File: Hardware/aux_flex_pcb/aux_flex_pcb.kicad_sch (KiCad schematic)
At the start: 17 parts, among them U1 STM32L432KCUx

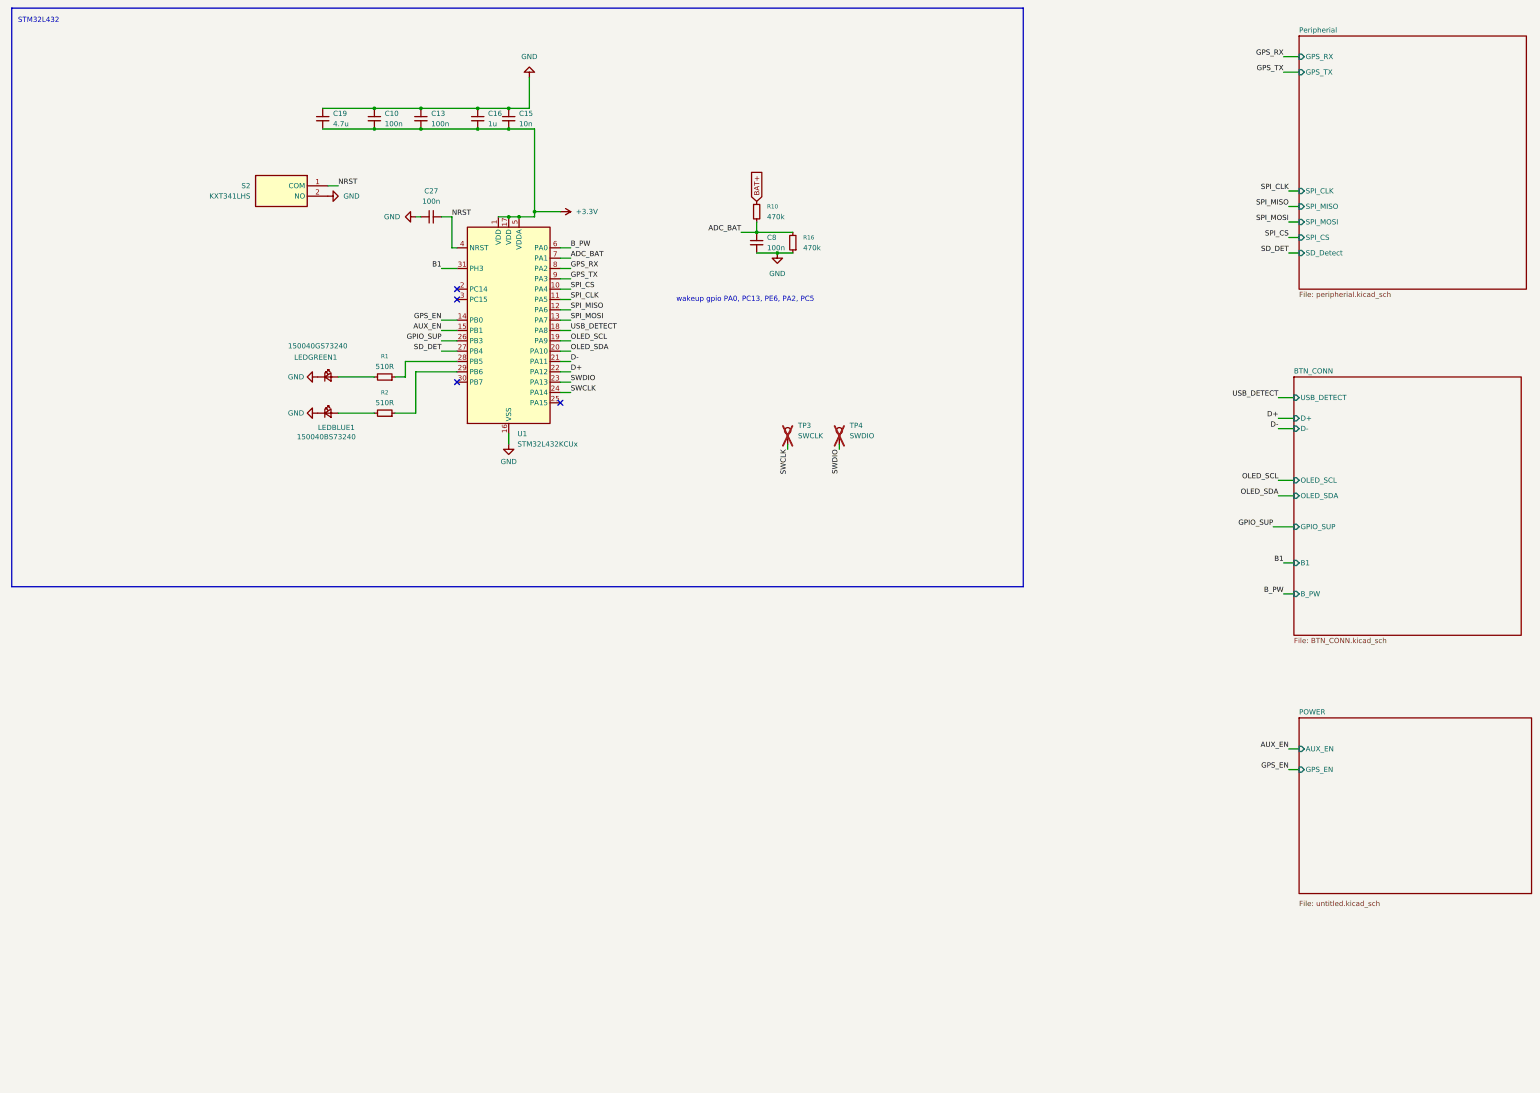
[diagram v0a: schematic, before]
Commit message: up
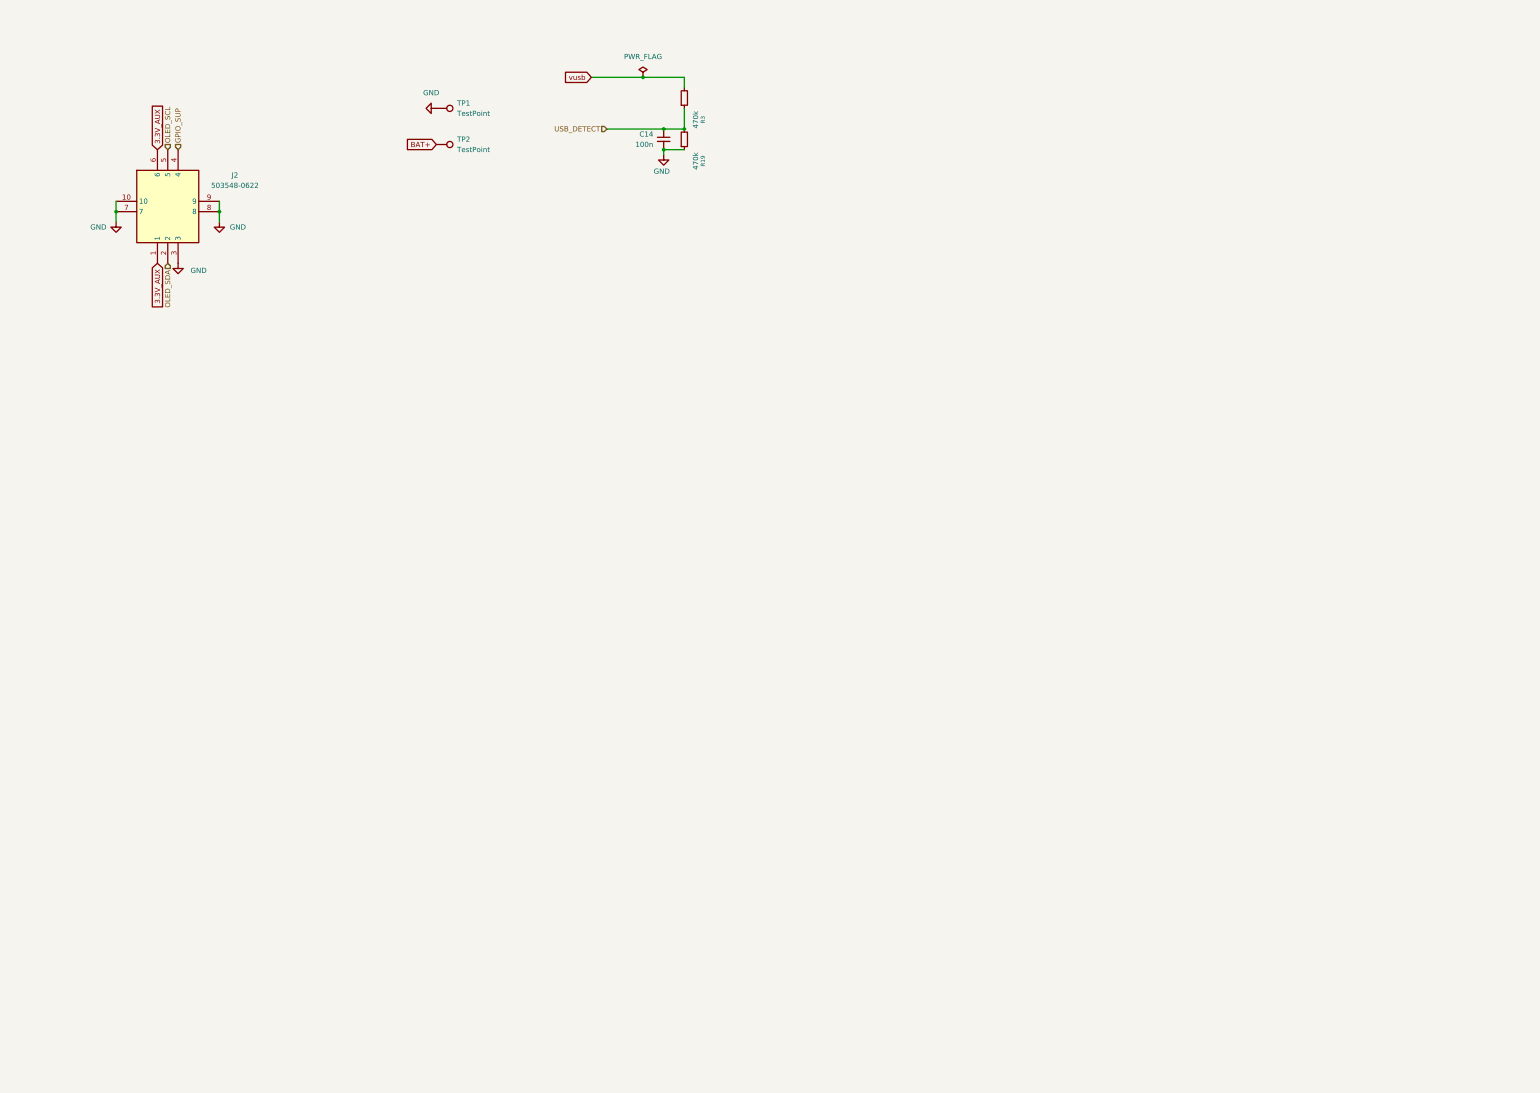
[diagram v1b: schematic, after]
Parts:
- removed C10, C13, C27, C8: 100n, v9footprint:C_0201_0603Metric_Pad0.64x0.40mm_HandSolder, symbol Device:C_Small
- removed C15: 10n, v9footprint:C_0201_0603Metric_Pad0.64x0.40mm_HandSolder, symbol Device:C_Small
- removed C16: 1u, v9footprint:C_0201_0603Metric_Pad0.64x0.40mm_HandSolder, symbol Device:C_Small
- removed C19: 4.7u, v9footprint:C_0402_1005Metric, symbol Device:C_Small
- removed LEDBLUE1: 150040BS73240, v9footprint:LED_0402_1005Metric, symbol Device:LED_Small
- removed LEDGREEN1: 150040GS73240, v9footprint:LED_0402_1005Metric, symbol Device:LED_Small
- removed R1, R2: 510R, v9footprint:R_0201_0603Metric_Pad0.64x0.40mm_HandSolder, symbol Device:R_Small
- removed R10, R16: 470k, v9footprint:R_0201_0603Metric_Pad0.64x0.40mm_HandSolder, symbol Device:R_Small
- removed S2: KXT341LHS, v9footprint:KXT341LHS, symbol samacsys:KXT341LHS
- removed TP3: SWCLK, v9footprint:pad_0.7mm, symbol Connector:TestPoint
- removed TP4: SWDIO, v9footprint:pad_0.7mm, symbol Connector:TestPoint
- removed U1: STM32L432KCUx, v9footprint:QFN-32-1EP_5x5mm_P0.5mm_EP3.45x3.45mm, symbol MCU_ST_STM32L4:STM32L432KCUx
- added C14: 100n, v9footprint:C_0201_0603Metric_Pad0.64x0.40mm_HandSolder, symbol Device:C_Small
- added J2: 503548-0622, v9footprint:5035480622, symbol samacsys2:503548-0622
- added R19, R3: 470k, v9footprint:R_0201_0603Metric_Pad0.64x0.40mm_HandSolder, symbol Device:R_Small
- added TP1, TP2: TestPoint, v9footprint:BAT_PAD_1mm, symbol Connector:TestPoint
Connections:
- net BAT+: now also TP2.1
- net GND: now also C14.2, J2.10, J2.3, J2.7, J2.8, J2.9, R19.1, TP1.1
- net GPIO_SUP: now also J2.4
- net OLED_SCL: now also J2.5
- net OLED_SDA: now also J2.2
- net USB_DETECT: now also C14.1, R19.2, R3.1
- new net 3.3V_AUX: J2.1, J2.6
- new net vusb: R3.2
- no-connect marks 4 -> 0
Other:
- removed sheet BTN_CONN
- removed sheet POWER
- removed sheet Peripherial
- note removed: "STM32L432"
- note removed: "wakeup gpio PA0, PC13, PE6, PA2, PC5"

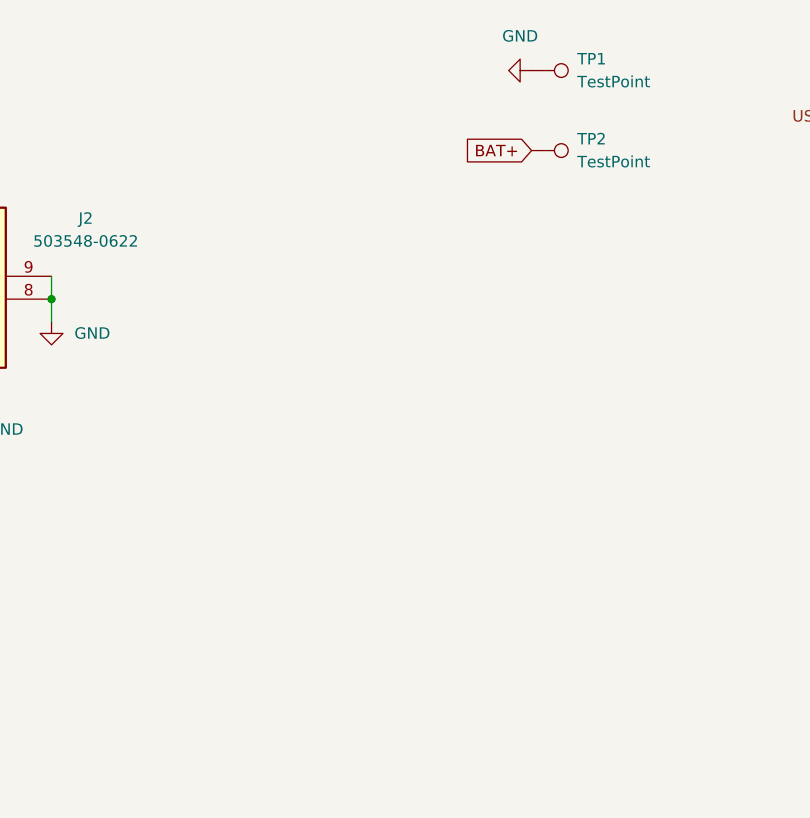
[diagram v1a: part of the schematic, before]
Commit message: up
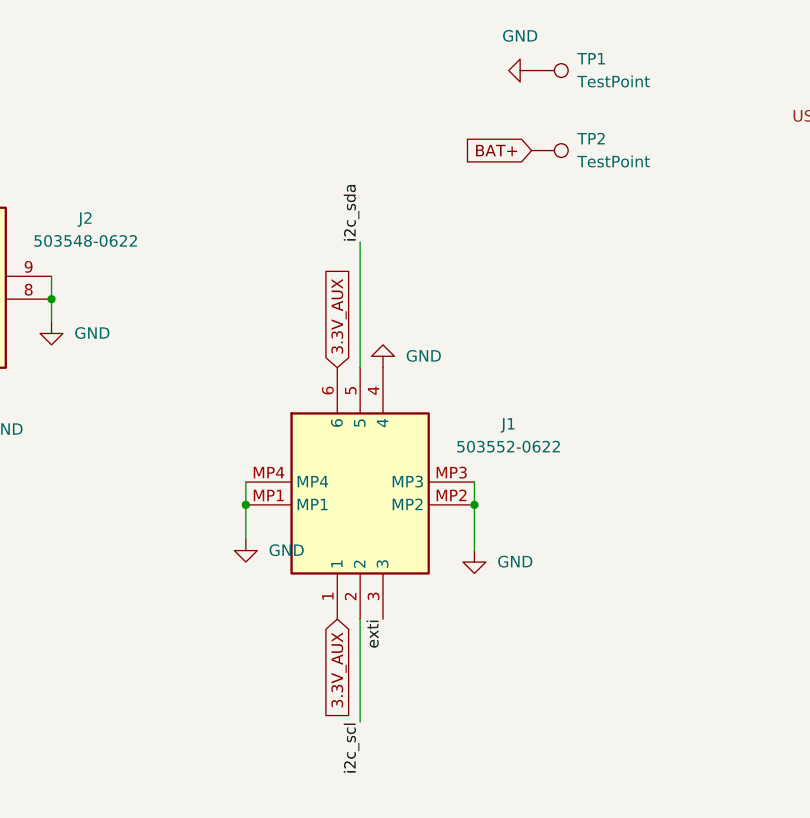
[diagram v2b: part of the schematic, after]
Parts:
- added J1: 503552-0622, samacsys2:5035520622, symbol samacsys2:503552-0622
- C14: footprint v9footprint:C_0201_0603Metric_Pad0.64x0.40mm_HandSolder -> Capacitor_SMD:C_0201_0603Metric_Pad0.64x0.40mm_HandSolder
- J2: footprint v9footprint:5035480622 -> samacsys2:5035480622
- R19, R3: footprint v9footprint:R_0201_0603Metric_Pad0.64x0.40mm_HandSolder -> Resistor_SMD:R_0201_0603Metric_Pad0.64x0.40mm_HandSolder
- TP1, TP2: footprint v9footprint:BAT_PAD_1mm -> samacsys2:1mm_circle
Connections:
- net 3.3V_AUX: now also J1.1, J1.6
- net GND: now also J1.4, J1.MP1, J1.MP2, J1.MP3, J1.MP4
- new net exti: J1.3
- new net i2c_scl: J1.2
- new net i2c_sda: J1.5

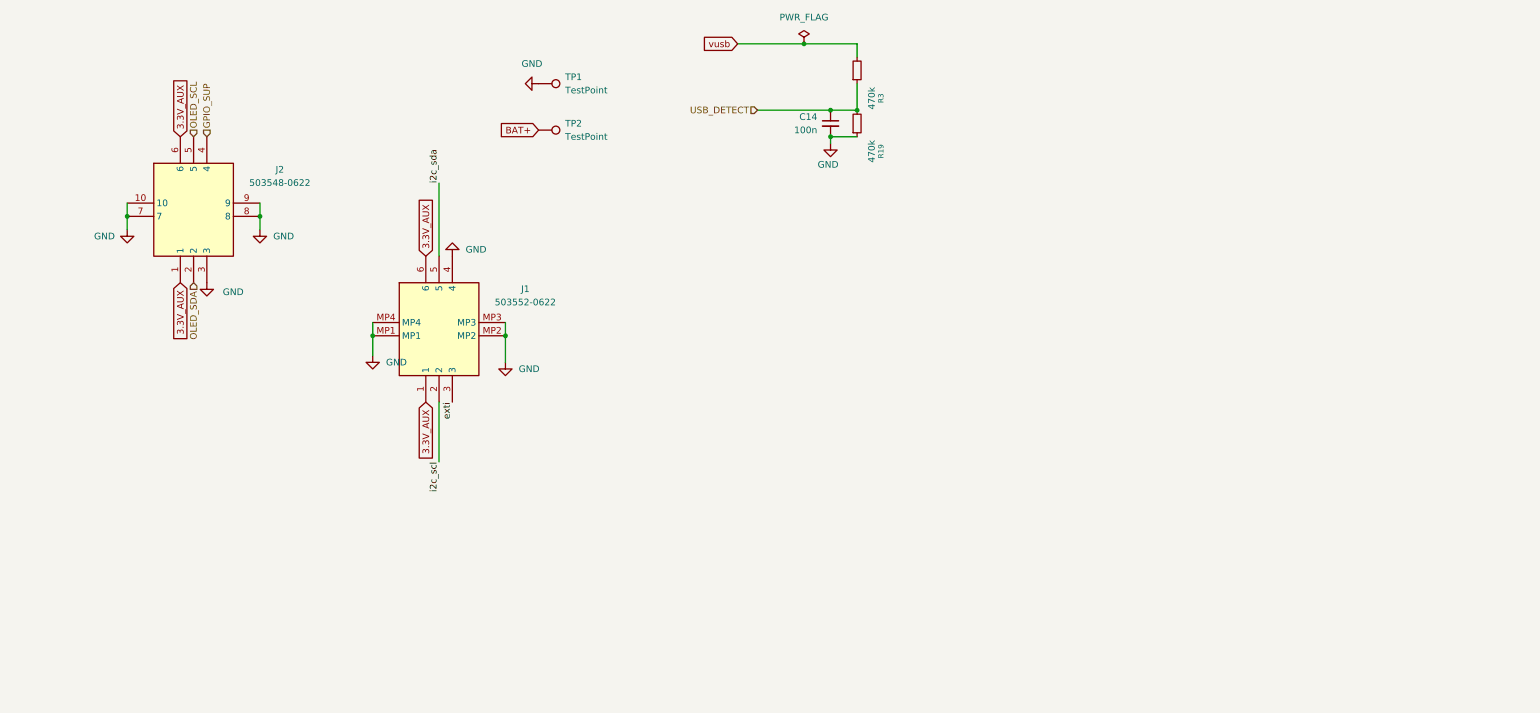
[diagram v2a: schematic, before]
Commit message: up
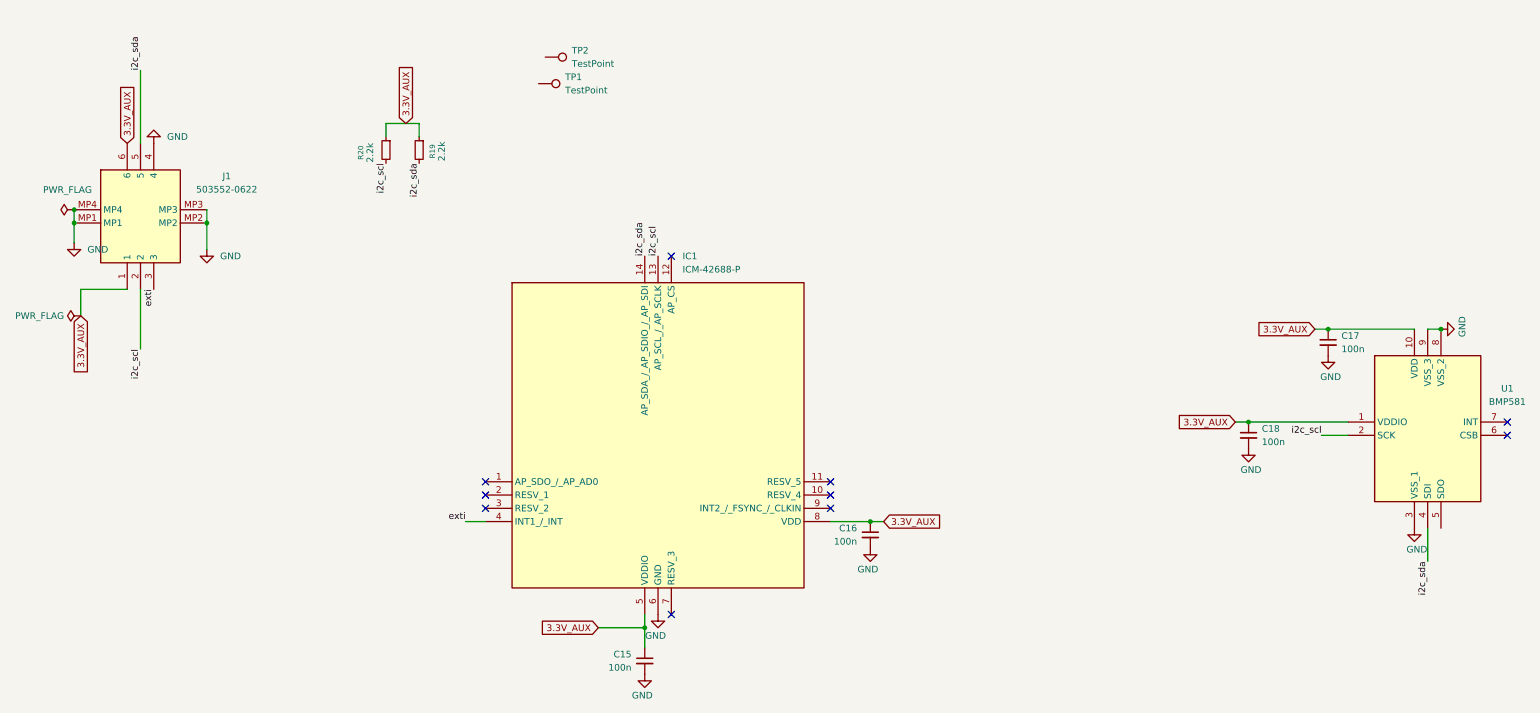
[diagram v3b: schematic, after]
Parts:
- removed C14: 100n, Capacitor_SMD:C_0201_0603Metric_Pad0.64x0.40mm_HandSolder, symbol Device:C_Small
- removed J2: 503548-0622, samacsys2:5035480622, symbol samacsys2:503548-0622
- removed R3: 470k, Resistor_SMD:R_0201_0603Metric_Pad0.64x0.40mm_HandSolder, symbol Device:R_Small
- added C15, C16, C17, C18: 100n, Capacitor_SMD:C_0201_0603Metric_Pad0.64x0.40mm_HandSolder, symbol Device:C_Small
- added IC1: ICM-42688-P, IIM42352, symbol samacsys:ICM-42688-P
- added R20: 2.2k, Resistor_SMD:R_0201_0603Metric_Pad0.64x0.40mm_HandSolder, symbol Device:R_Small
- added U1: BMP581, BMP581, symbol samacsys:BMP581
- R19: value 470k -> 2.2k
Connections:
- net USB_DETECT is gone; now on net i2c_sda: R19.2
- net 3.3V_AUX: now also R19.1, C15.1, C16.1, C17.1, C18.1, IC1.5 (VDDIO), IC1.8 (VDD), R20.1, U1.1 (VDDIO), U1.10 (VDD)
- net GND: now also C15.2, C16.2, C17.2, C18.2, IC1.6 (GND), U1.3 (VSS_1), U1.8 (VSS_2), U1.9 (VSS_3); no longer R19.1, TP1.1
- net exti: now also IC1.4 (INT1_/_INT)
- net i2c_scl: now also IC1.13 (AP_SCL_/_AP_SCLK), R20.2, U1.2 (SCK)
- net i2c_sda: now also IC1.14 (AP_SDA_/_AP_SDIO_/_AP_SDI), U1.4 (SDI)
- net BAT+: no longer names the net of TP2.1
- no-connect marks 0 -> 10
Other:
- moved on the sheet: J1, R19, TP2
